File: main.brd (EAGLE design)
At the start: 76.2 x 63.5 mm, 48 parts, among them J1 PJ-015AH-SMT-TR, J3 1734510-1, U1 ATMEGA328P-AU, U2 DRV8833PWPR, U3 LS7366R-TS, U4 LP38691DTX-5.0/NOPB, U5 FT232RL-REEL, Y1 16MHz, Y2 30MHz

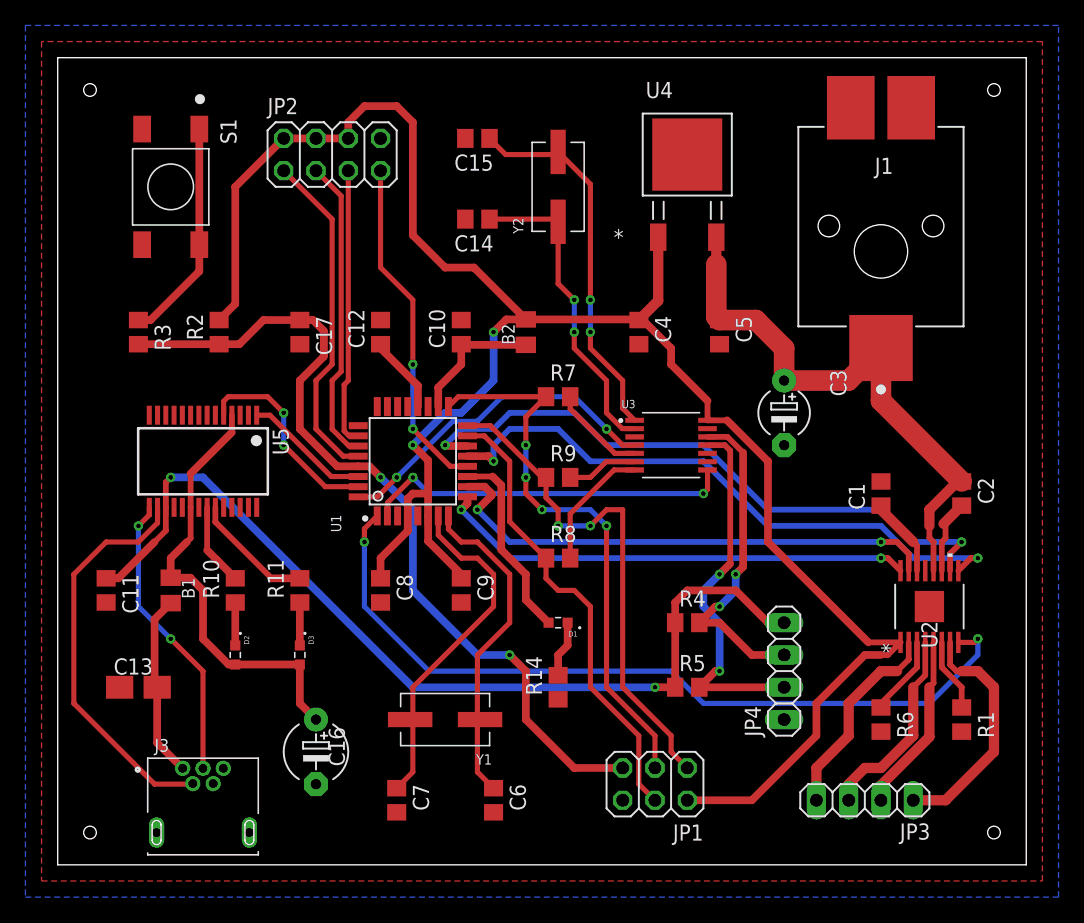
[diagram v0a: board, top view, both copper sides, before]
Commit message: Add files via upload
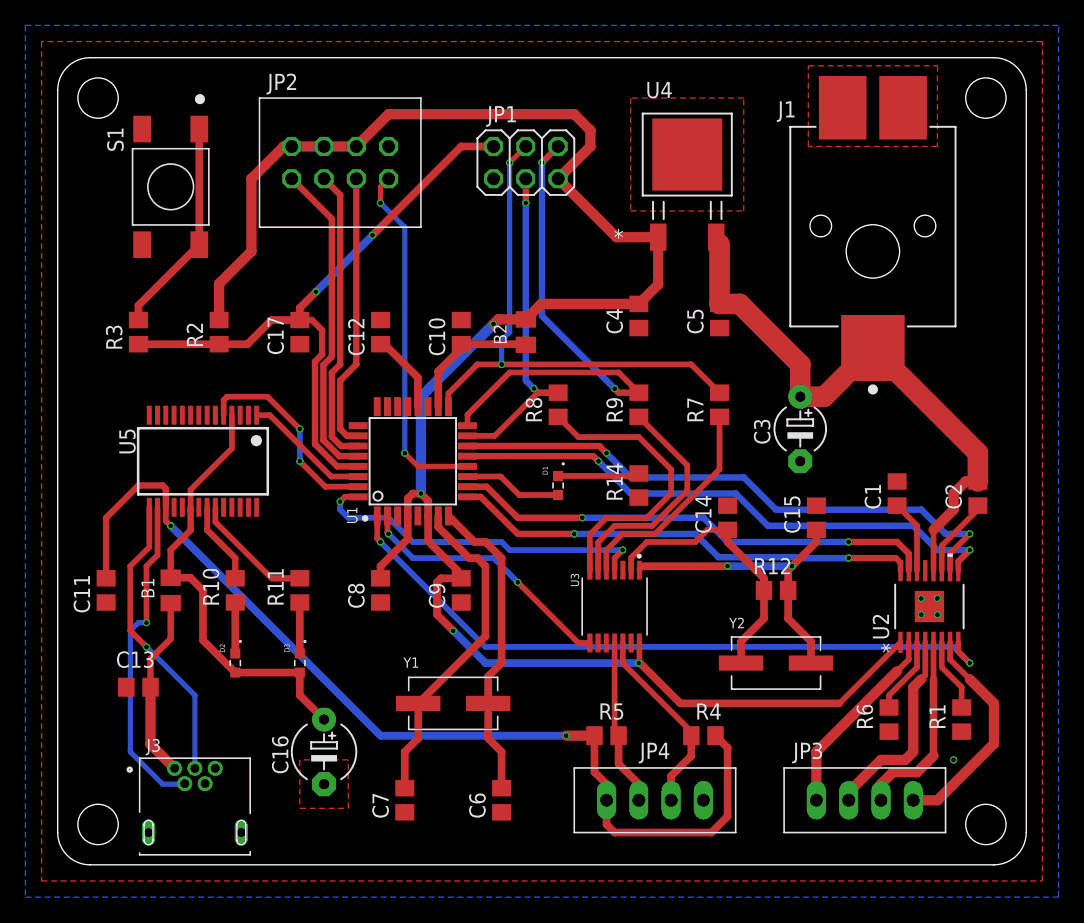
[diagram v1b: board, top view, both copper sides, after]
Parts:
- added R12: 1M, rcl:R0805
- C13: device rcl:A/3216-18W -> rcl:C0805
- JP2: device pinhead:2X04 -> Downloads:2X04
- JP3, JP4: device pinhead:1X04 -> Downloads:1X04
- moved JP1 49.9 mm to (36.8, 55.2)
- moved Y2 41.2 mm to (56.5, 15.9), turned to 0 degrees
- moved C15 40.0 mm to (59.7, 27.3), turned to 90 degrees
- moved C14 30.7 mm to (52.7, 27.3), turned to 90 degrees
- moved R14 17.1 mm to (45.7, 29.8)
- moved JP4 14.4 mm to (47.0, 5.08), turned to 180 degrees
- moved U3 13.5 mm to (43.8, 20.3), turned to 270 degrees
- moved R7 12.7 mm to (52.1, 36.2), turned to 270 degrees
- moved R8 12.1 mm to (39.4, 36.2), turned to 270 degrees
- moved D1 10.8 mm to (39.4, 29.8), turned to 270 degrees
- moved R4 8.98 mm to (50.8, 10.2), turned to 180 degrees
- moved R9 8.54 mm to (45.7, 36.2), turned to 270 degrees
- moved R5 7.41 mm to (43.2, 10.2)
- moved C3 1.80 mm to (58.4, 34.3)
- moved Y1 1.42 mm to (31.1, 12.7)
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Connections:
- removed net ENCA: JP4.3, R4.2, U3.12
- removed net ENCB: JP4.2, R5.2, U3.11
- new net N$7: JP4.3, R5.2, U3.11
- new net N$8: JP4.2, R4.2, U3.12
- net FCKI: now also R12.2
- net FCKO: now also R12.1
- net GND: now also C13.2; no longer C13.-
- net VCC: now also C13.1; no longer C13.+
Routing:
- net ENCB: track 29.5 -> 0.00 mm, vias 2 -> 0
- net ENCA: track 26.0 -> 0.00 mm, vias 2 -> 0
- net !RESET!: track 72.6 -> 50.3 mm
- net N$8: track 0.00 -> 15.3 mm
- net N$7: track 0.00 -> 13.2 mm
- net MO: track 9.99 -> 23.0 mm
- net MI: track 5.59 -> 18.3 mm
- net SCLK: track 7.48 -> 17.2 mm
- net !FAULT!: track 63.5 -> 54.5 mm
- net MOSI: track 36.3 -> 27.3 mm, vias 0 -> 2
- net LFLAG: track 29.2 -> 20.8 mm
- net +5V: track 161.5 -> 153.6 mm, vias 2 -> 4
- net N$5: track 15.3 -> 7.73 mm
- net N$9: track 31.6 -> 25.8 mm, vias 0 -> 1
- net FCKO: track 29.6 -> 24.3 mm
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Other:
- outline, holes or cut-outs redrawn
